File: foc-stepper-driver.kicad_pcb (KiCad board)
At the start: 4 copper layers, 42 x 42 mm, 72 parts, among them CN1 C42391660, CN2 C2839706, CN3 C2839705, CN4 C2839704, J2 TC2030, U1 DRV8962DDWR, U2 TYPE-C 16PLT-H10.0, U3 STM32G431CBT6, U6 AS5047P-ATSM, U7 TPS560430XDBVR, U8 SPX3819M5-L-3-3/TR, U9 TCAN3403DRQ1, X1 NX3215SA 32.768KHZ EXS00A-MU0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, X2 NDK NX2016SA-24MHZ-EXS00A-CS1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

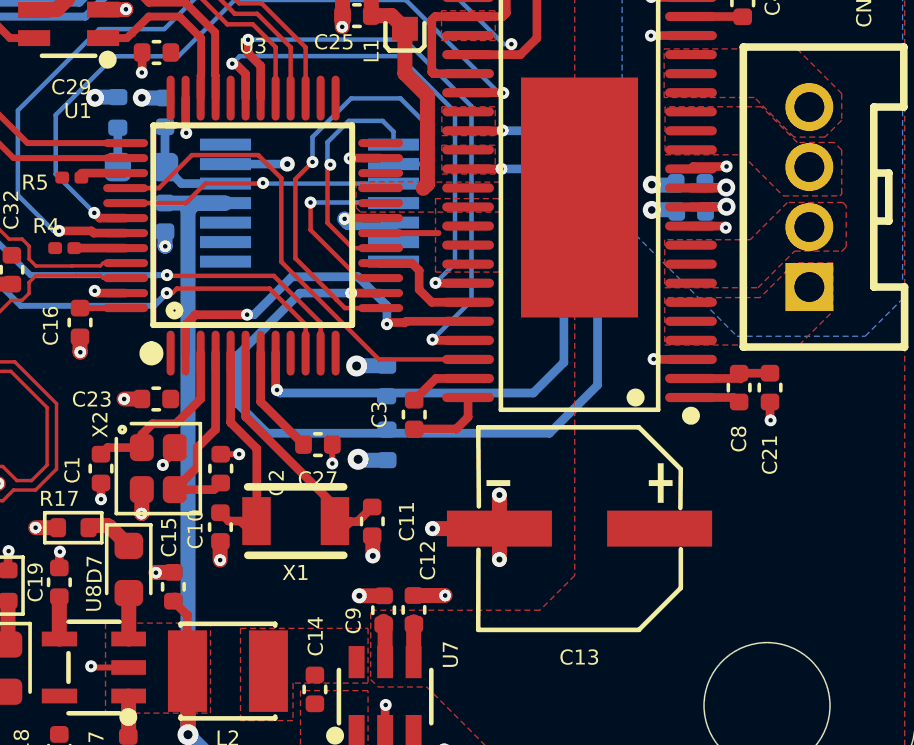
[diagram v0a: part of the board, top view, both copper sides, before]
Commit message: update
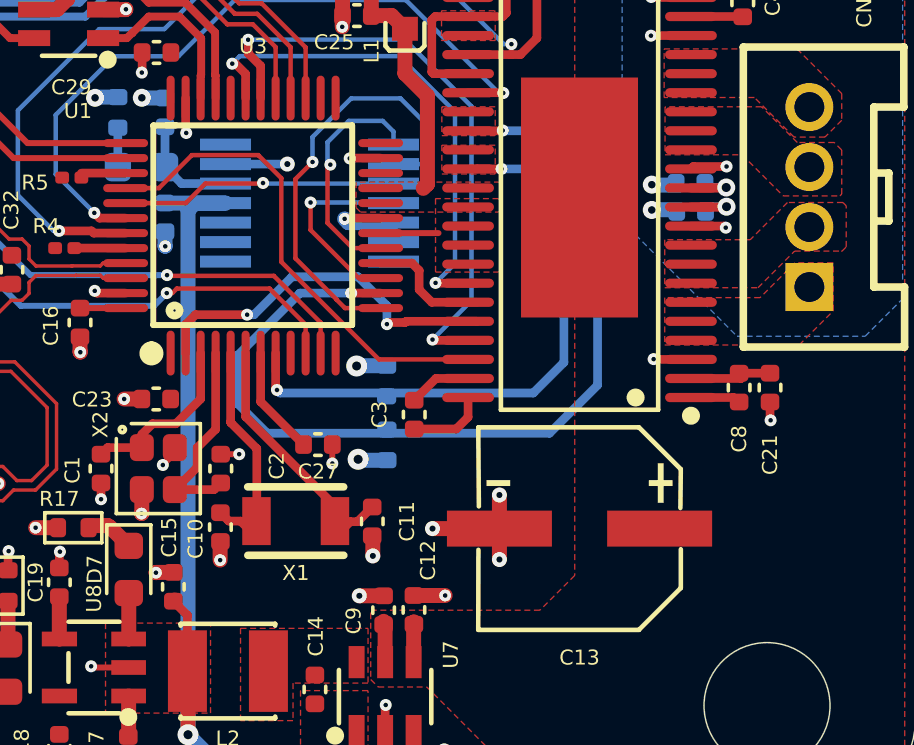
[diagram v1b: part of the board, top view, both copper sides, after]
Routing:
- net +24V: vias 4 -> 2
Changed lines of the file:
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@@
 		(tags "capacitor")
 		(property "Reference" "C10"
-			(at 0.07 0.83 90)
+			(at 0.39 0.83 90)
 			(layer "F.SilkS")
 			(effects
@@
 		(tags "capacitor")
 		(property "Reference" "C27"
-			(at 0 -1.16 0)
+			(at 0 -0.9 0)
 			(layer "F.SilkS")
 			(effects
@@
 		(tags "capacitor")
 		(property "Reference" "C2"
-			(at -0.47 1.87 90)
+			(at 0.09 1.87 90)
 			(layer "F.SilkS")
 			(effects
@@
 	(via
 		(at 149.95 83.87)
-		(size 0.5)
-		(drill 0.2)
-		(layers "F.Cu" "B.Cu")
-		(net 6)
-	)
-	(via
-		(at 149.95 83.87)
 		(size 0.6)
 		(drill 0.3)
@@
 		(net 6)
 	)
-	(via
-		(at 149.94 83.23)
-		(size 0.5)
-		(drill 0.2)
-		(layers "F.Cu" "B.Cu")
-		(net 6)
-	)
 	(segment
 		(start 149.32 84.04)
@@
 			(thermal_gap 0.5)
 			(thermal_bridge_width 0.5)
-			(smoothing fillet)
-			(radius 2)
 		)
 		(polygon
